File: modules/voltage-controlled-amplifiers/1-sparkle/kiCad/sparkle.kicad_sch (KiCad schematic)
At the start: 83 parts, among them J1 OUT_1, J2 IN_1, J3 CV_1, J4 OUT_2, J5 IN_2, J6 CV_2, Q1 BC548, Q2 BC548, Q3 BC548, Q4 BC548, U1 TL074

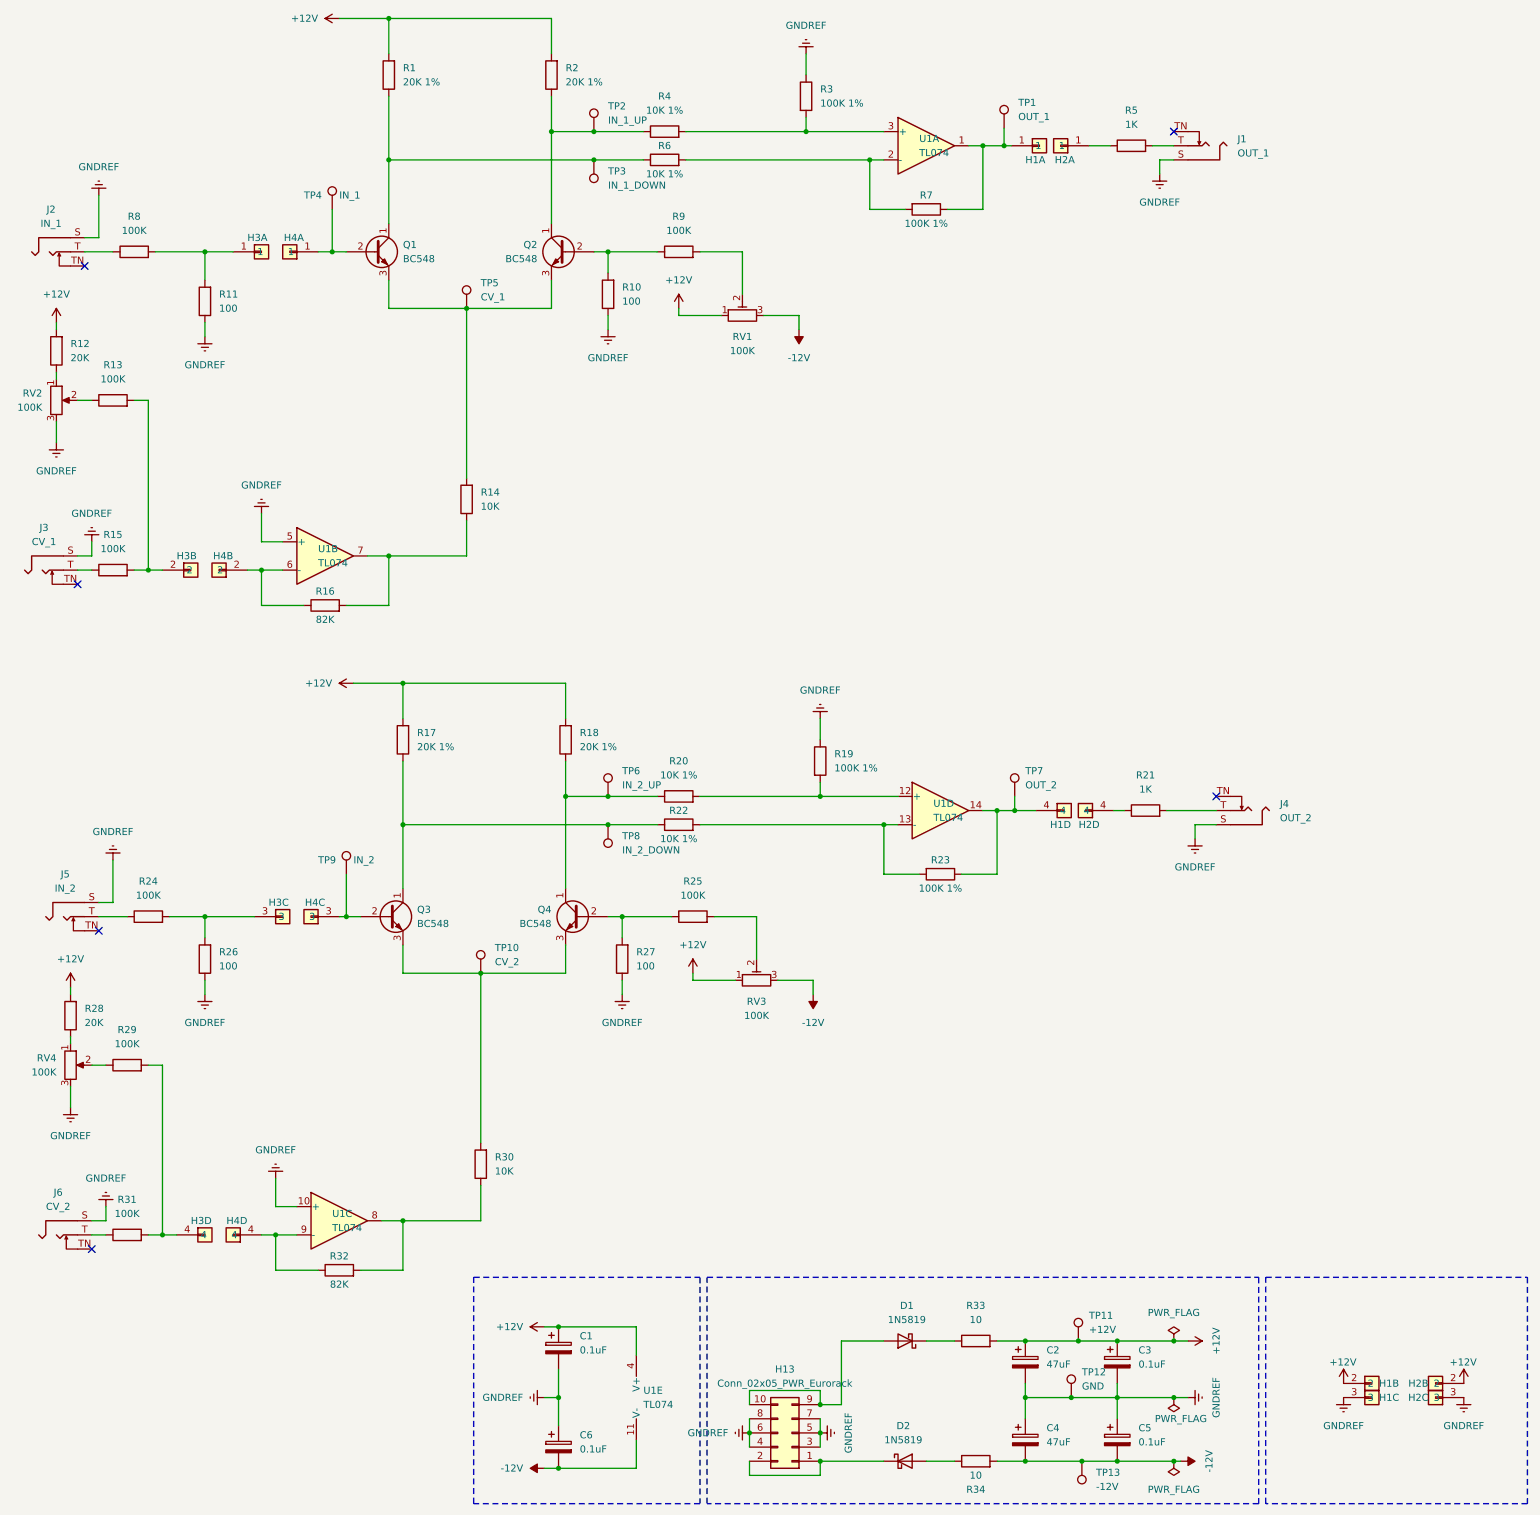
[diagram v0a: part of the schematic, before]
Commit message: update pcbs and symbols
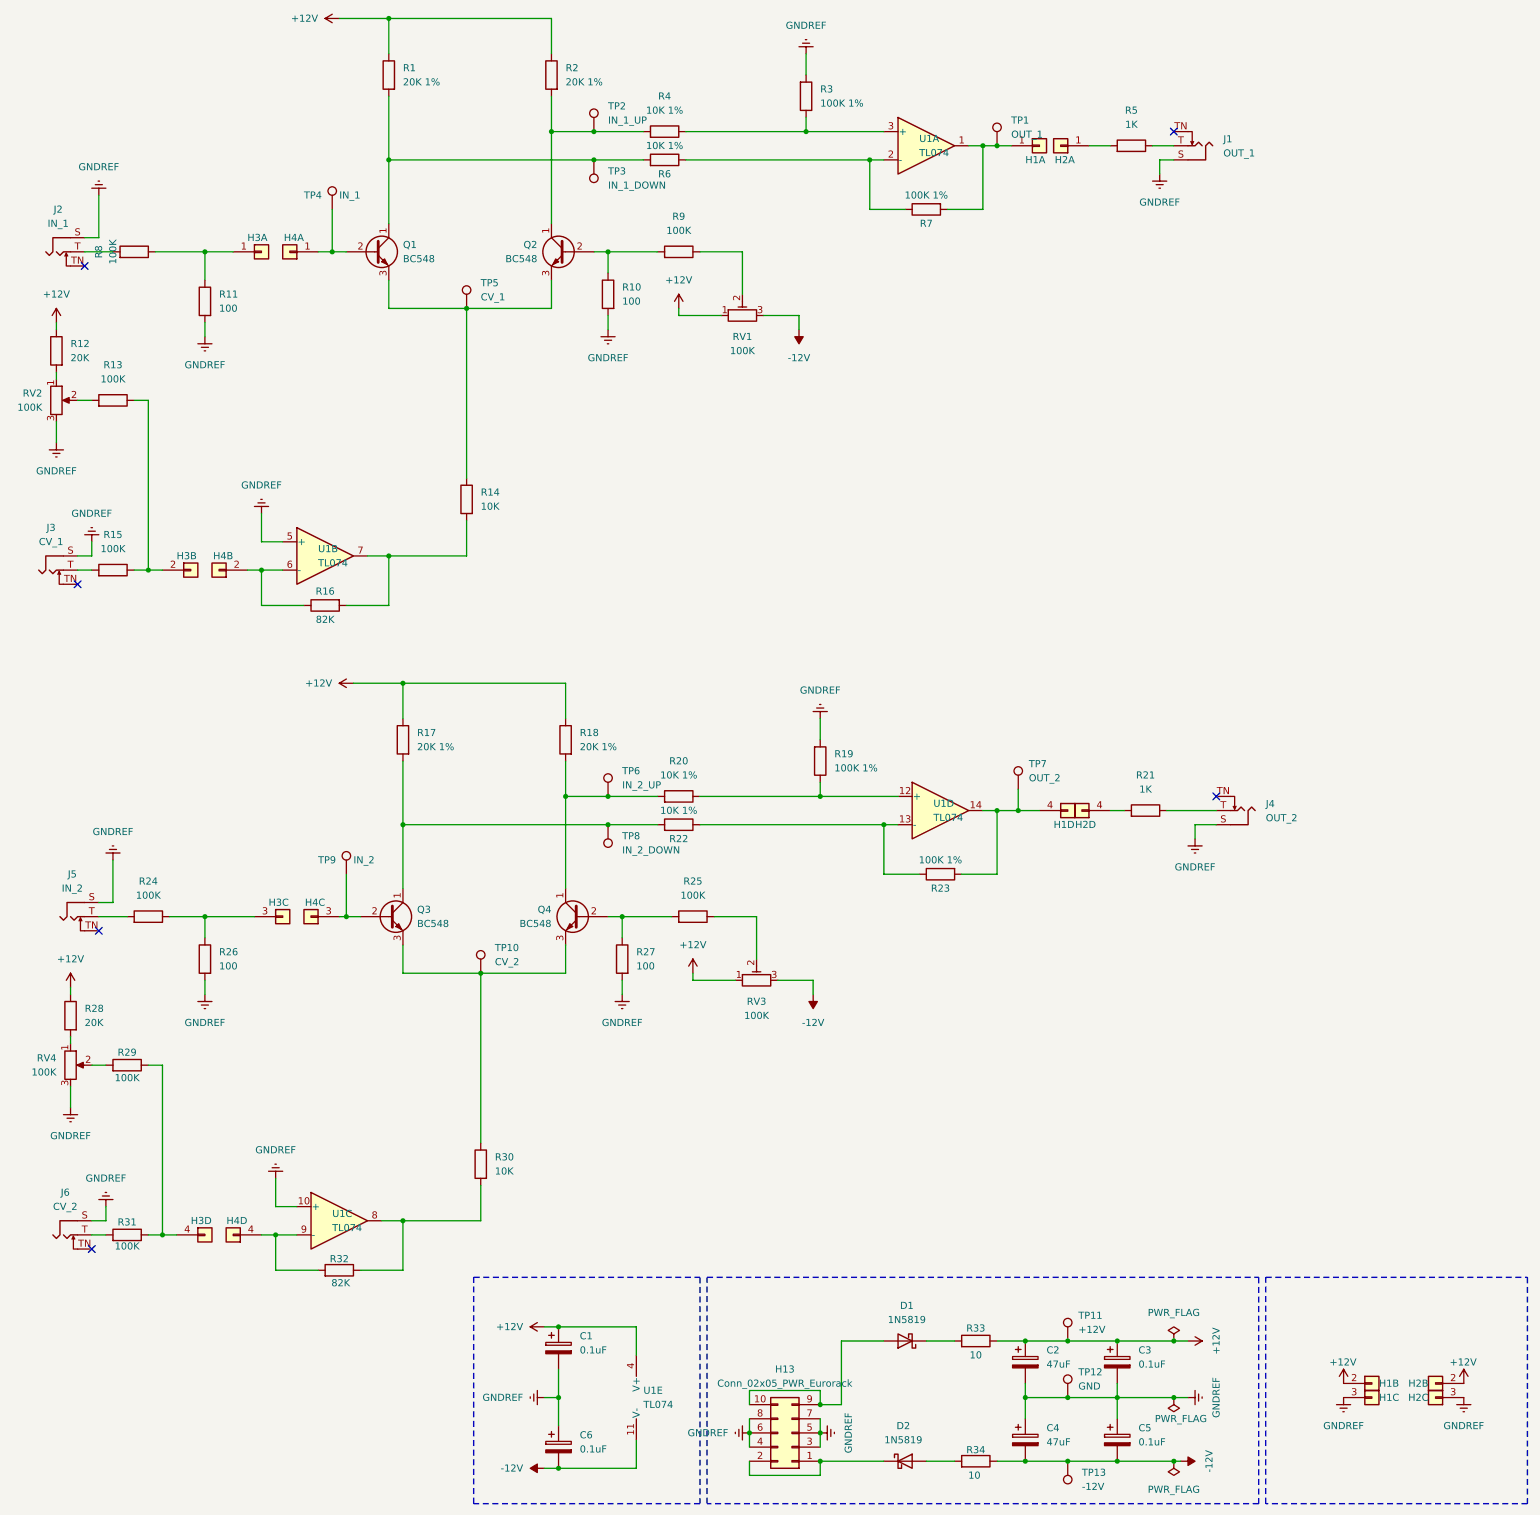
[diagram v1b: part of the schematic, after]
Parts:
- D1, D2: footprint synth-custom:D_PWR_default -> Synth:D_DO-41_SOD81_P10.16mm_Horizontal; symbol Diode:1N5819 -> synth:D_Schottky (1N5819)
- H1, H4: footprint synth-custom:PinSocket_1x04_P2.54mm_Vertical -> Synth:PinSocket_1x04_P2.54mm_Vertical; symbol Synth_Custom:CONN_Socket_01x04 -> synth:PinSocket_01x04
- H13: footprint synth-custom:CONN_02x05_PWR -> Synth:IDC-Header_2x05_P2.54mm_Vertical; symbol Synth_Custom:CONN_02x05_PWR_Eurorack -> synth:Conn_02x05_EuroRack_Power
- H2, H3: footprint synth-custom:PinHeader_1x04_P2.54mm_Vertical -> Synth:PinHeader_1x04_P2.54mm_Vertical; symbol Synth_Custom:CONN_Header_01x04 -> synth:PinHeader_01x04
- J1, J2, J3, J4, J5, J6: footprint synth-custom:Jack_default -> Connector_Audio:Jack_3.5mm_QingPu_WQP-PJ398SM_Vertical_CircularHoles; symbol Synth_Custom:Jack_default -> synth:AudioJack_Mono_3.5mm
- R1, R10, R11, R12, R13, R14, R15, R16, R17, R18, R19, R2, R20, R21, R22, R23, R24, R25, R26, R27, R28, R29, R3, R30, R31, R32, R33, R34, R4, R5, R6, R7, R8, R9: footprint synth-custom:R_default -> Synth:R_Default (DIN0207); symbol Device:R -> synth:R_Default
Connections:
- net at R14.1, U1.7: now also R16.1; no longer R16.2
- net at H4.2 (Pin_2), U1.6 (-): now also R16.2; no longer R16.1
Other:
- moved on the sheet: J1, J2, J3, J4, J5, J6, R1, R10, R11, R12, R13, R14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
